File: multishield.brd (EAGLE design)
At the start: 57.6 x 53.7 mm, 21 parts, among them J1 7p-2.54-90d, J2 2x16p-2.54, J3 7p-2.54-90d, J4 2x6p-2.54, J5 7p-2.54-90d, J6 7p-2.54-90d, K2 TS-1101F, M1 ARDUINO_R3_ICSP, SW1 SK-12D01, U1 AD595AQ-DIP14, U2 ATMEGA328P_PDIP, Y1 16MHZ

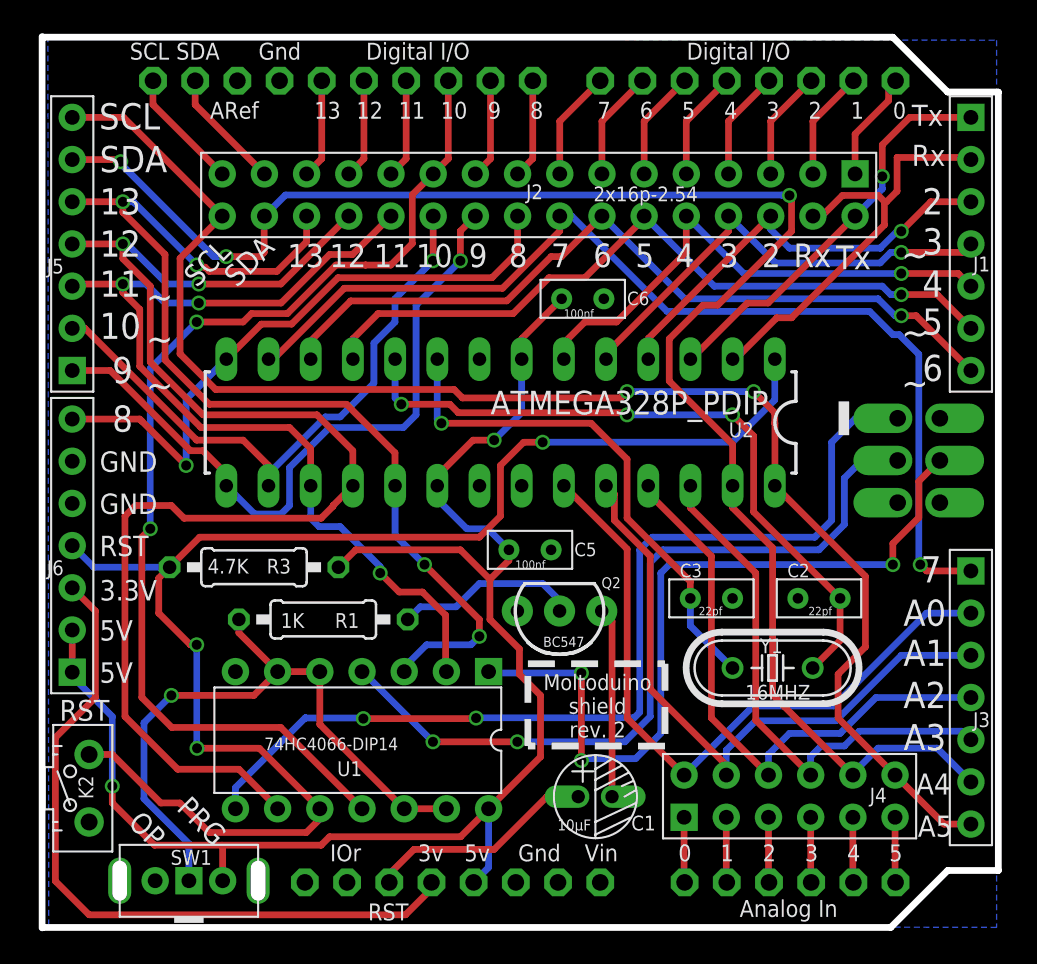
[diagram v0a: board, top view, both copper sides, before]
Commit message: various improvements and addition of LED at D9
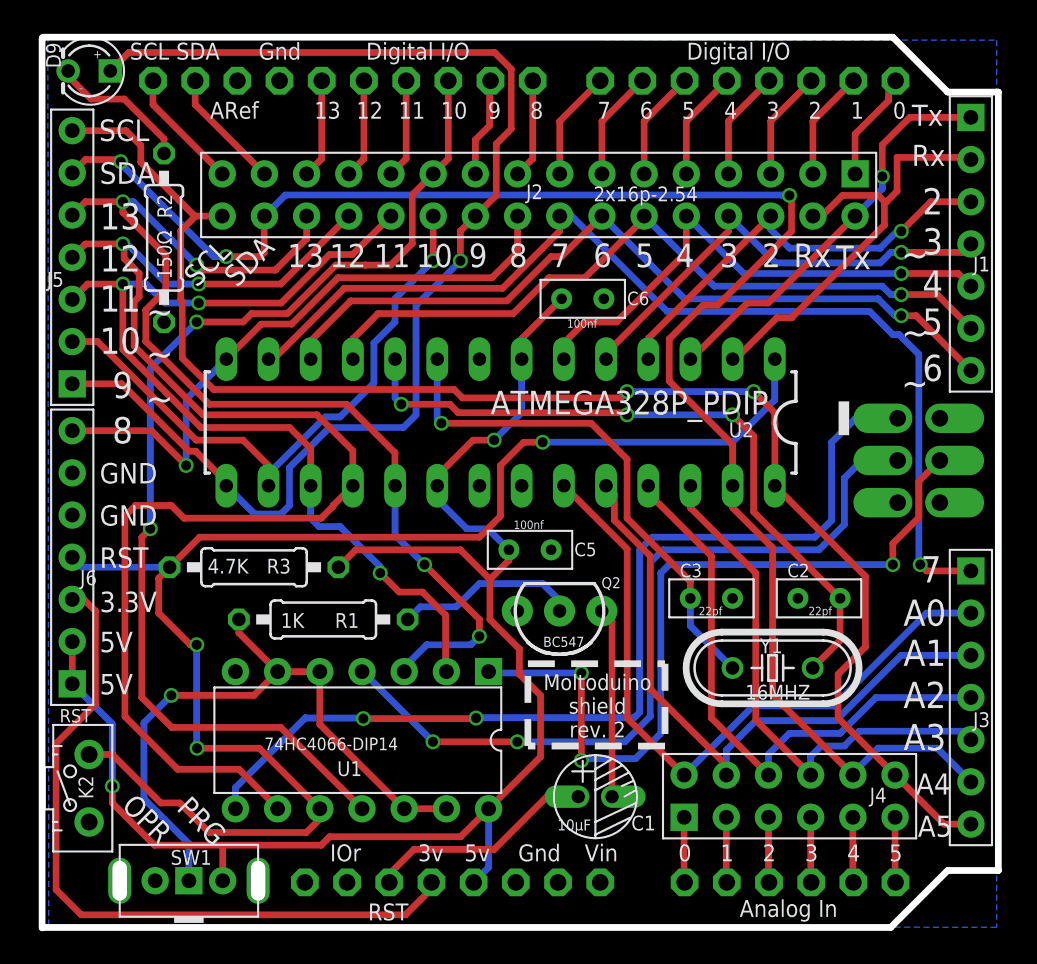
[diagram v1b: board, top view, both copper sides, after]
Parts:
- added D9: SR302DC, Seeed-OPL-Diode:LED2-2.54-D3.0MM
- added R2: 150Ω, Seeed-OPL-Resistor:PR-D2.3XL6.5MM
- moved J5 0.80 mm to (4.57, 40.5)
- moved J6 0.70 mm to (4.57, 22.4)
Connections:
- net N$18 renamed D9A
- removed net N$34: J2.23, J5.1, U2.15
- new net D9B: D9.A, J2.23, J5.1, U2.15
- new net N$18: D9.K, R2.1
- net GND: now also R2.2
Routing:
- net D9B: track 0.00 -> 76.1 mm, vias 0 -> 1
- net N$34: track 41.9 -> 0.00 mm, vias 1 -> 0
- net N$18: track 0.00 -> 8.53 mm
- net SCK: track 63.6 -> 64.7 mm
- net VCC: track 93.3 -> 92.6 mm
- net MISO: track 82.4 -> 83.0 mm
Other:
- board size 57.6 x 53.7 mm -> 57.6 x 53.6 mm
- board text added: "OPR"
- board text removed: "OP"
